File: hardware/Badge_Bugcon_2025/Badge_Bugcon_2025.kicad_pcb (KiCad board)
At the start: 2 copper layers, 100 x 100 mm, 162 parts, among them J1 Conn_01x21, J10 Battery, J13 ETH, J14 Conn_01x23, J4 USB_A, J5 Conn_01x22, J6 USB_A, J7 Add_On, J8 Conn_01x23, J9 Add_On, P4 USB_C_Plug_USB2.0, Q1 DMG3415U-7, SW1 ON, SW2 SW_Push, SW3 SW_Push, SW4 USB Selector, U1 FSUSB30MUX, U2 TP4056, U3 SL2.1A, U4 MT3608, U5 AP2114H-3.3, U6 W25N02KVZEIR, U7 EA3059, Y1 Crystal, Y2 24MHz, Y5 Crystal_GND2

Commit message: fix(hw): route pads
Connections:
- C31 pad 1: VCC -> +5V
- U5 pad 3: VCC -> +5V

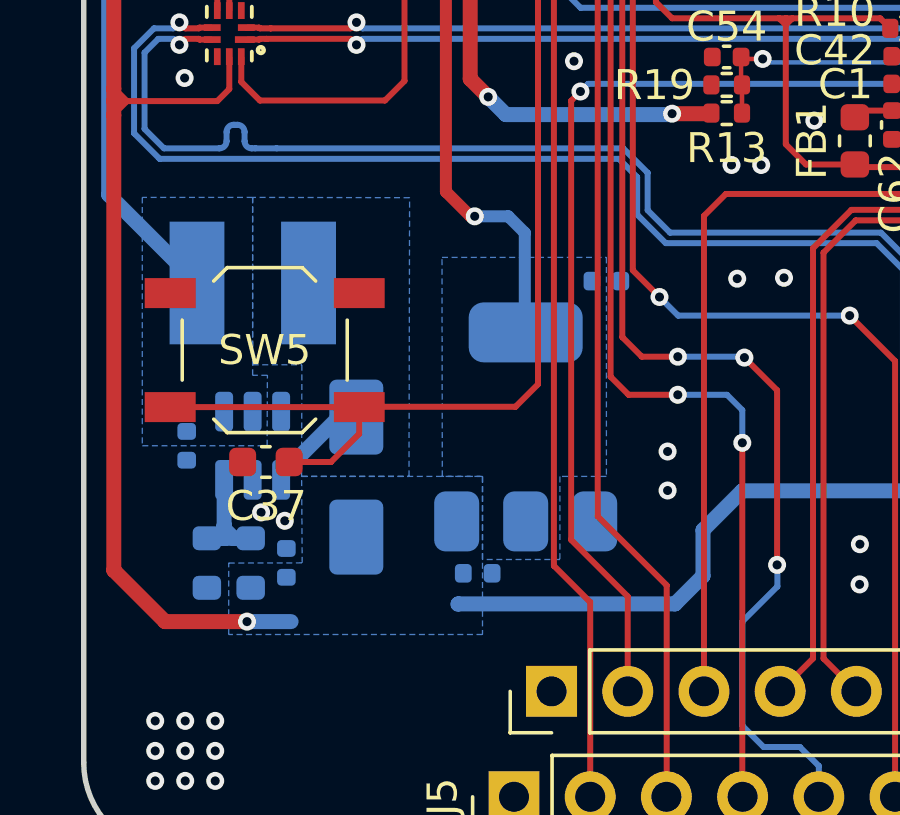
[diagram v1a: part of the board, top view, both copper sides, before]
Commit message: feat(Hw):Update_Route
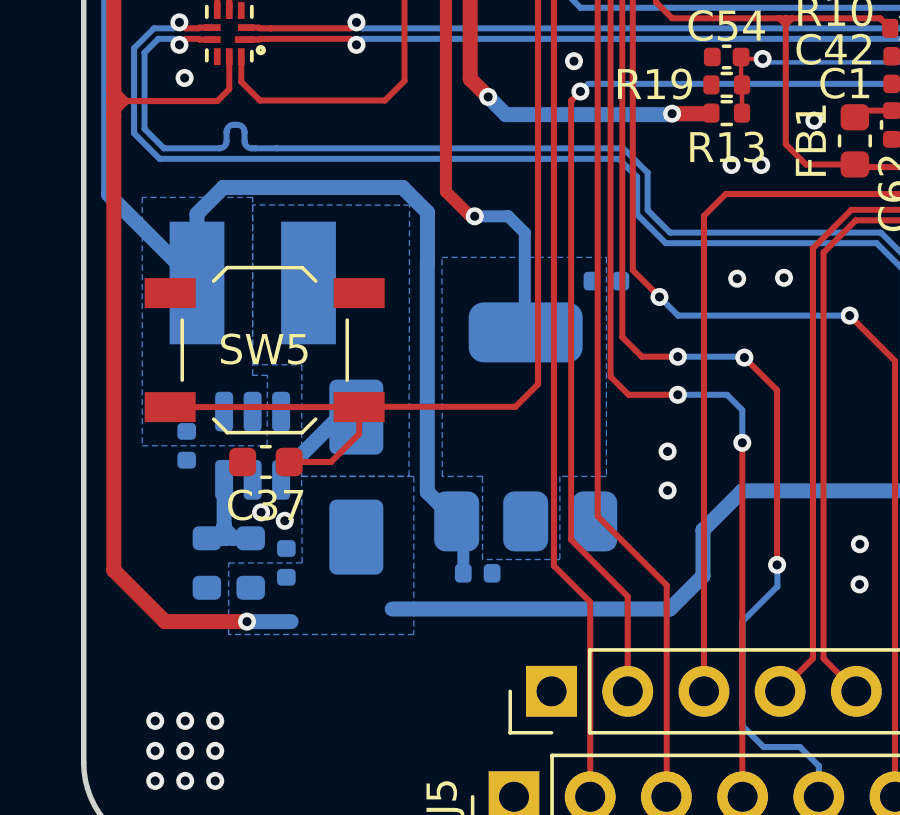
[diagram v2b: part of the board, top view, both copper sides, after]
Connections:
- C31 pad 1: +5V -> VCC
- U5 pad 3: +5V -> VCC
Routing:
- net VCC: track 195.3 -> 218.6 mm
- net +5V: track 196.0 -> 198.3 mm
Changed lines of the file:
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@@
 			(layers "B.Cu" "B.Mask" "B.Paste")
 			(roundrect_rratio 0.25)
-			(net 73 "+5V")
+			(net 13 "VCC")
 			(pintype "passive")
 		)
@@
 			(layers "B.Cu" "B.Mask" "B.Paste")
 			(roundrect_rratio 0.25)
-			(net 73 "+5V")
+			(net 13 "VCC")
 			(pinfunction "VIN")
 			(pintype "power_in")
@@
 	)
 	(segment
+		(start 113.16 119.89)
+		(end 113.16 118.38)
+		(width 0.4)
+		(layer "B.Cu")
+		(net 13)
+	)
+	(segment
 		(start 123.242235 76.565319)
 		(end 123.242235 76.397819)
@@
 	)
 	(segment
+		(start 104.2835 110.213096)
+		(end 104.2835 107.9065)
+		(width 0.5)
+		(layer "B.Cu")
+		(net 13)
+	)
+	(segment
+		(start 111.965 107.855)
+		(end 111.965 109.52)
+		(width 0.5)
+		(layer "B.Cu")
+		(net 13)
+	)
+	(segment
 		(start 122.42 76.097819)
 		(end 122.942235 76.097819)
@@
 	)
 	(segment
+		(start 111.14 107.03)
+		(end 111.965 107.855)
+		(width 0.5)
+		(layer "B.Cu")
+		(net 13)
+	)
+	(segment
 		(start 116.19 67.6)
 		(end 113.56 67.6)
@@
 	)
 	(segment
+		(start 111.96 109.525)
+		(end 111.96 117.18)
+		(width 0.5)
+		(layer "B.Cu")
+		(net 13)
+	)
+	(segment
 		(start 123.242235 75.645319)
 		(end 123.242235 76.565319)
@@
 	)
 	(segment
+		(start 111.965 109.52)
+		(end 111.96 109.525)
+		(width 0.5)
+		(layer "B.Cu")
+		(net 13)
+	)
+	(segment
 		(start 120.812235 80.195319)
 		(end 119.742235 79.125319)
@@
 	)
 	(segment
+		(start 113.16 118.38)
+		(end 112.94 118.16)
+		(width 0.4)
+		(layer "B.Cu")
+		(net 13)
+	)
+	(segment
 		(start 120.892235 72.210319)
 		(end 119.742235 73.360319)
@@
 	)
 	(segment
+		(start 105.16 107.03)
+		(end 111.14 107.03)
+		(width 0.5)
+		(layer "B.Cu")
+		(net 13)
+	)
+	(segment
+		(start 111.96 117.18)
+		(end 112.94 118.16)
+		(width 0.5)
+		(layer "B.Cu")
+		(net 13)
+	)
+	(segment
 		(start 116.019735 80.340319)
 		(end 116.017235 80.342819)
@@
 	)
 	(segment
+		(start 104.2835 107.9065)
+		(end 105.16 107.03)
+		(width 0.5)
+		(layer "B.Cu")
+		(net 13)
+	)
+	(segment
 		(start 113.56 67.6)
 		(end 103.3 67.6)
@@
 	)
 	(segment
-		(start 122.459 117.141)
-		(end 121.15 118.45)
+		(start 121.15 118.45)
+		(end 121.15 119.98)
 		(width 0.5)
 		(layer "B.Cu")
@@
 	)
 	(segment
+		(start 120.05 121.08)
+		(end 110.79 121.08)
+		(width 0.5)
+		(layer "B.Cu")
+		(net 73)
+	)
+	(segment
 		(start 152.74 117.131)
 		(end 152.75 117.141)
@@
 	)
 	(segment
-		(start 120.22 120.91)
-		(end 112.99 120.91)
+		(start 121.15 119.98)
+		(end 120.05 121.08)
 		(width 0.5)
 		(layer "B.Cu")
@@
 	)
 	(segment
-		(start 164.89 104.71)
-		(end 164.89 102.91)
+		(start 122.459 117.141)
+		(end 121.15 118.45)
 		(width 0.5)
 		(layer "B.Cu")
@@
 	)
 	(segment
-		(start 164.337765 105.262235)
-		(end 164.89 104.71)
+		(start 152.12 117.141)
+		(end 122.459 117.141)
 		(width 0.5)
 		(layer "B.Cu")
@@
 	)
 	(segment
-		(start 152.74 116.46)
-		(end 152.74 117.131)
+		(start 164.89 104.71)
+		(end 164.89 102.91)
 		(width 0.5)
 		(layer "B.Cu")
@@
 	)
 	(segment
-		(start 167.35 102.11)
-		(end 167.35 102.14)
+		(start 164.337765 105.262235)
+		(end 164.89 104.71)
 		(width 0.5)
 		(layer "B.Cu")
@@
 	)
 	(segment
-		(start 112.99 120.91)
-		(end 112.98 120.92)
+		(start 152.74 116.46)
+		(end 152.74 117.131)
 		(width 0.5)
 		(layer "B.Cu")
@@
 	)
 	(segment
-		(start 121.15 118.45)
-		(end 121.15 119.98)
+		(start 167.35 102.11)
+		(end 167.35 102.14)
 		(width 0.5)
 		(layer "B.Cu")
@@
 	)
 	(segment
-		(start 152.12 117.141)
-		(end 122.459 117.141)
-		(width 0.5)
-		(layer "B.Cu")
-		(net 73)
-	)
-	(segment
 		(start 162.164681 105.262235)
 		(end 164.337765 105.262235)
@@
 	)
 	(segment
-		(start 121.15 119.98)
-		(end 120.22 120.91)
-		(width 0.5)
-		(layer "B.Cu")
-		(net 73)
-	)
-	(segment
 		(start 167.35 102.14)
 		(end 168.03 101.46)
@@
 		(polygon
 			(pts
-				(xy 107.77 116.66) (xy 111.35 116.66) (xy 111.37 107.37) (xy 106.1375 107.36) (xy 106.1375 112.94)
+				(xy 107.77 116.66) (xy 111.35 116.66) (xy 111.369462 107.62) (xy 106.1375 107.610001) (xy 106.1375 112.94)
 				(xy 107.78 112.94)
 			)
@@
 		(polygon
 			(pts
-				(xy 105.34 119.548096) (xy 107.79 119.543096) (xy 107.77 116.66) (xy 113.8 116.66) (xy 113.8 121.93)
+				(xy 105.34 119.548096) (xy 107.79 119.543096) (xy 107.77 116.66) (xy 111.51 116.66) (xy 111.51 121.93)
 				(xy 105.34 121.93) (xy 105.34 119.543096)
 			)
